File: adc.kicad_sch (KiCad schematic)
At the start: 14 parts, among them U4 PCM1860DBT, U6 STM32F401RBTx, Y1 12.288MHz

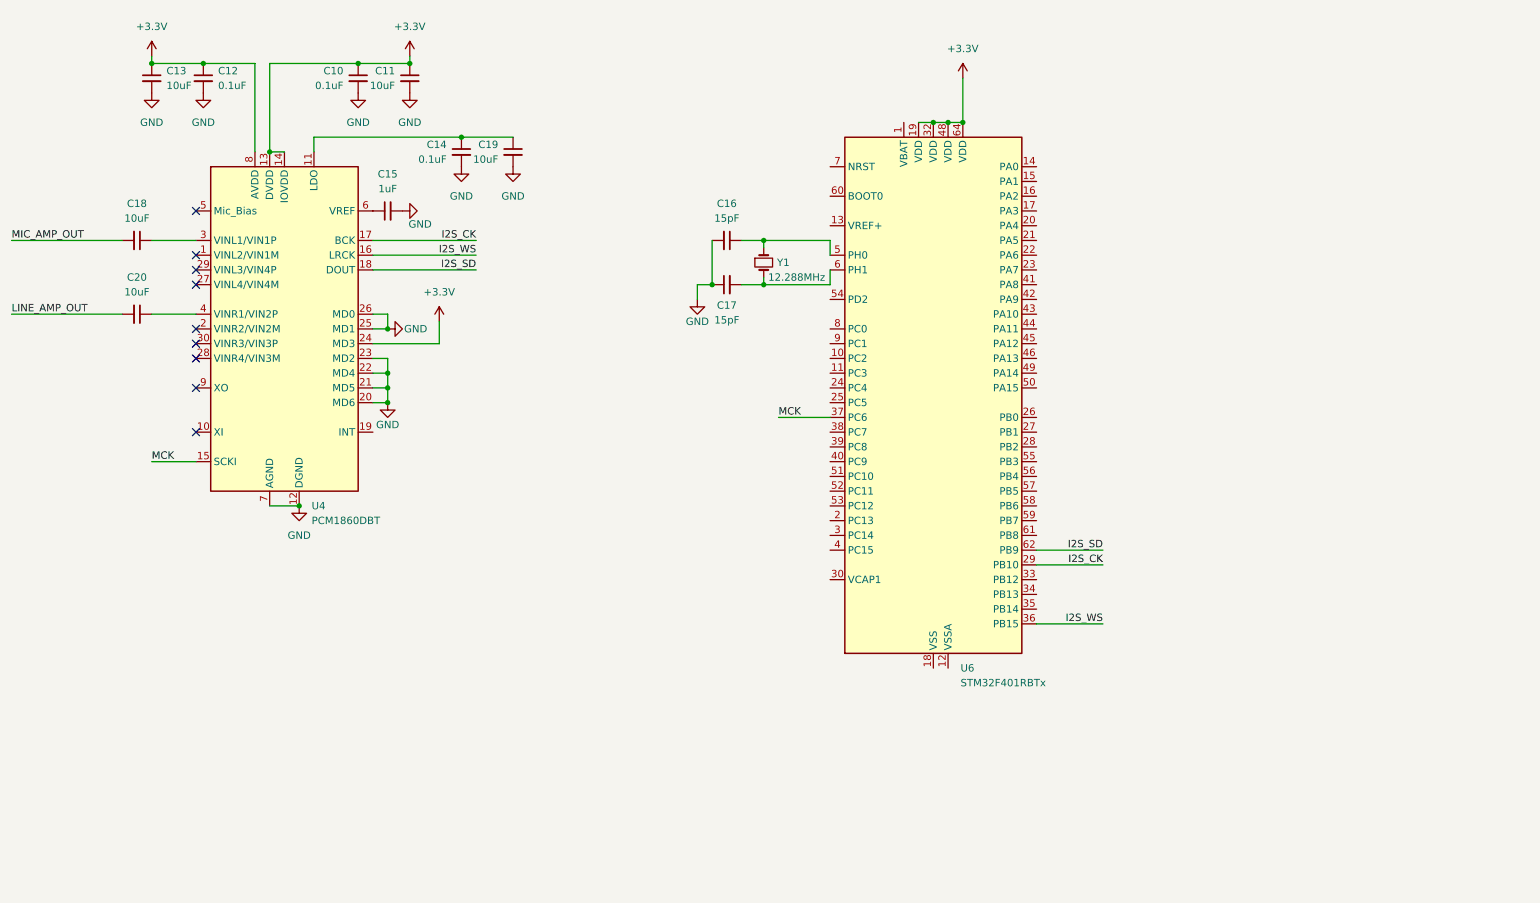
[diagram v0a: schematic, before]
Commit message: wow... just wow...
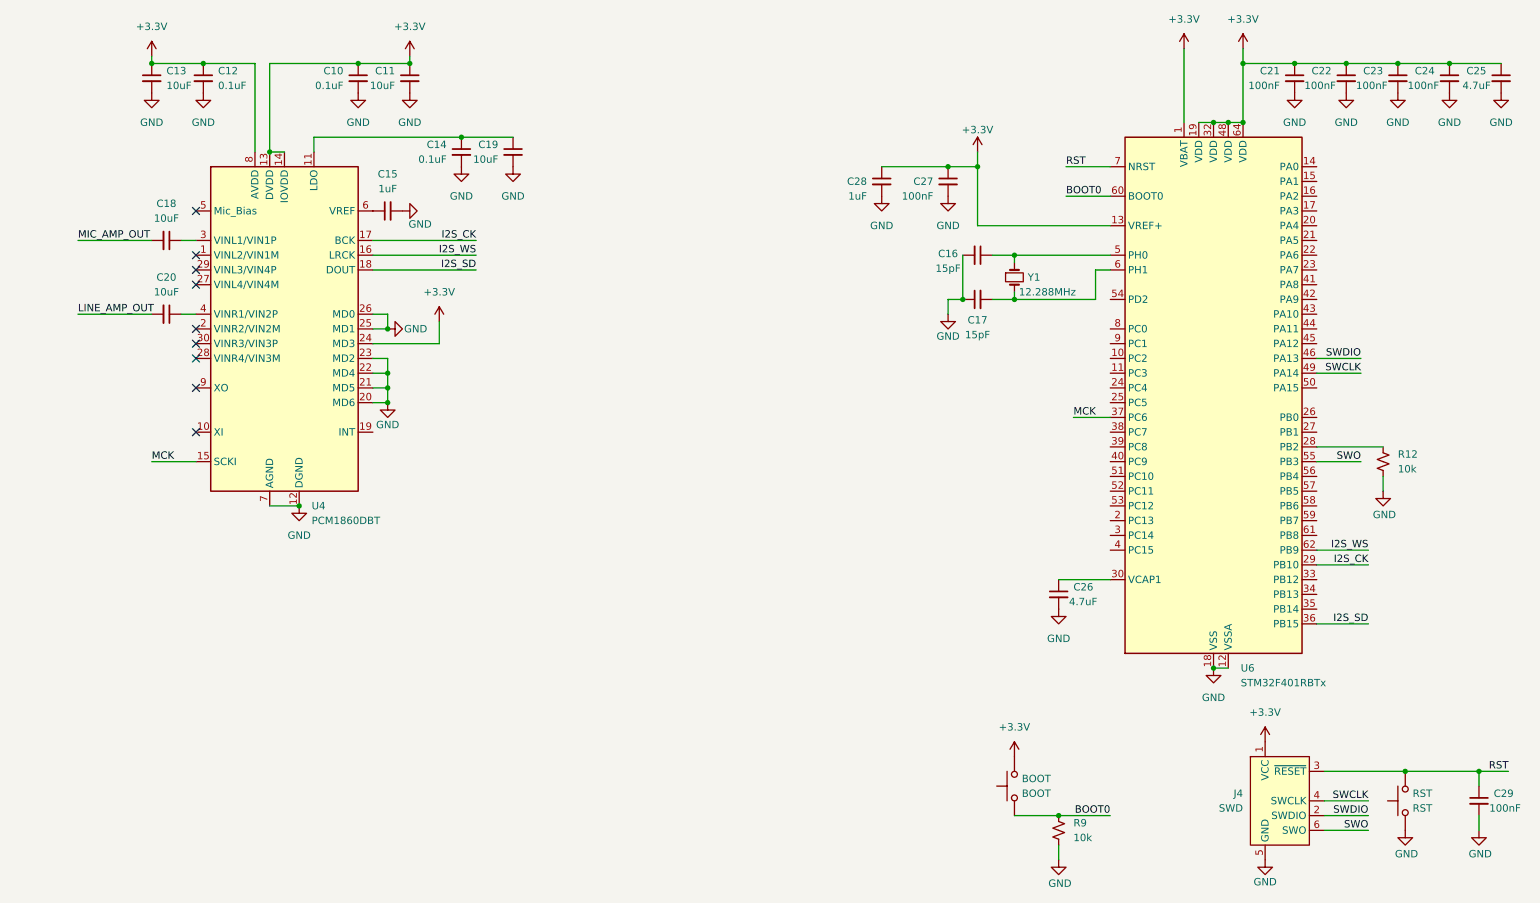
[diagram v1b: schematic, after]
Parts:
- added BOOT: BOOT, symbol Switch:SW_Push
- added C21, C22, C23, C24, C27, C29: 100nF, symbol Device:C_Small
- added C25, C26: 4.7uF, symbol Device:C_Small
- added C28: 1uF, symbol Device:C_Small
- added J4: SWD, Connector:Tag-Connect_TC2030-IDC-NL_2x03_P1.27mm_Vertical, symbol Connector:Conn_ARM_SWD_TagConnect_TC2030-NL
- added R12, R9: 10k, symbol Device:R_Small_US
- added RST: RST, symbol Switch:SW_Push
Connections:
- net +3.3V: now also U6.1 (VBAT), U6.13 (VREF+), BOOT.2, C21.1, C22.1, C23.1, C24.1, C25.1, C27.1, C28.1, J4.1 (VCC)
- net GND: now also U6.12 (VSSA), U6.18 (VSS), U6.31 (VSS), U6.47 (VSS), U6.63 (VSS), C21.2, C22.2, C23.2, C24.2, C25.2, C26.2, C27.2, C28.2, C29.2, J4.5 (GND), R12.2, R9.2, RST.1
- net I2S_SD: now also U6.36 (PB15); no longer U6.62 (PB9)
- net I2S_WS: now also U6.62 (PB9); no longer U6.36 (PB15)
- net at U6.28 (PB2): now also R12.1
- net at U6.30 (VCAP1): now also C26.1
- net SWDIO: now reaches U6.46 (PA13)
- net SWDIO: now also J4.2 (SWDIO)
- net SWCLK: now reaches U6.49 (PA14)
- net SWCLK: now also J4.4 (SWCLK)
- net SWO: now reaches U6.55 (PB3)
- net SWO: now also J4.6 (SWO)
- net BOOT0: now reaches U6.60 (BOOT0)
- net BOOT0: now also BOOT.1, R9.1
- net RST: now reaches U6.7 (NRST)
- net RST: now also C29.1, J4.3 (~{RESET}), RST.2
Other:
- moved on the sheet: C16, C17, C18, C20, U6, Y1
